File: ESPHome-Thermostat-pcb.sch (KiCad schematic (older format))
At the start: 97 parts, among them J1 Si7021, J2 MT3608, J3 Relay_Out, J4 SSD1306_Display, J5 Vin, Q1 NMOS_YJL03N06A, Q10 PMOS_AP40P05, Q11 NMOS_YJL03N06A, Q12 PMOS_AP40P05, Q13 PMOS_AP40P05, Q14 NMOS_YJL03N06A, Q15 NMOS_YJL03N06A, Q16 PMOS_AP40P05, Q17 NMOS_YJL03N06A, Q18 PMOS_AP40P05, Q19 PMOS_AP40P05, Q2 NMOS_YJL03N06A, Q20 PMOS_AP40P05, Q3 PMOS_AP40P05, Q4 PMOS_AP40P05, Q5 NMOS_YJL03N06A, Q6 NMOS_YJL03N06A, Q7 PMOS_AP40P05, Q8 PMOS_AP40P05, Q9 NMOS_YJL03N06A, SW1 EC11_Rotary_Encoder_Switch, U1 NodeMCU_1.0_(ESP-12E), U2 PCF8574, U3 AMS1117-3.3

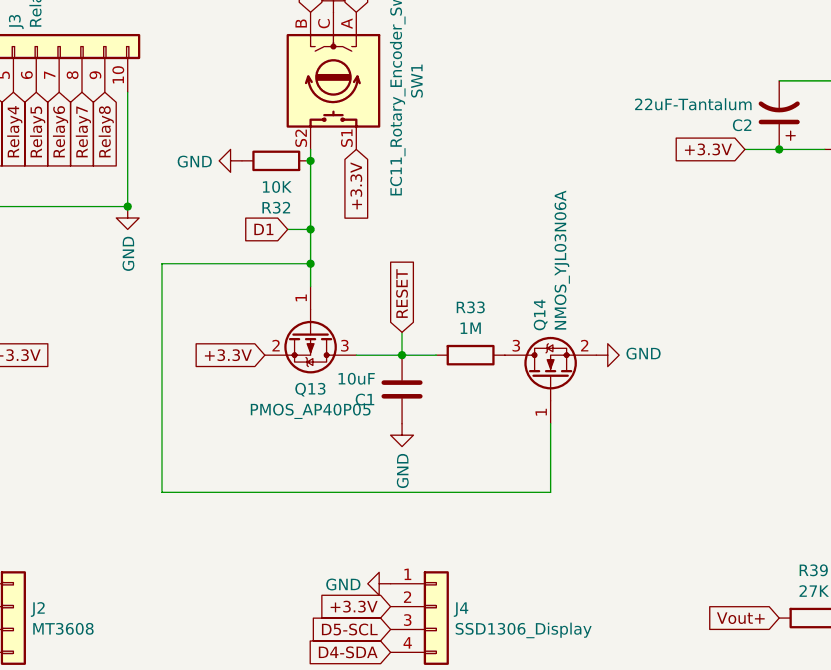
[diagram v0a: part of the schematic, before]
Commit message: development
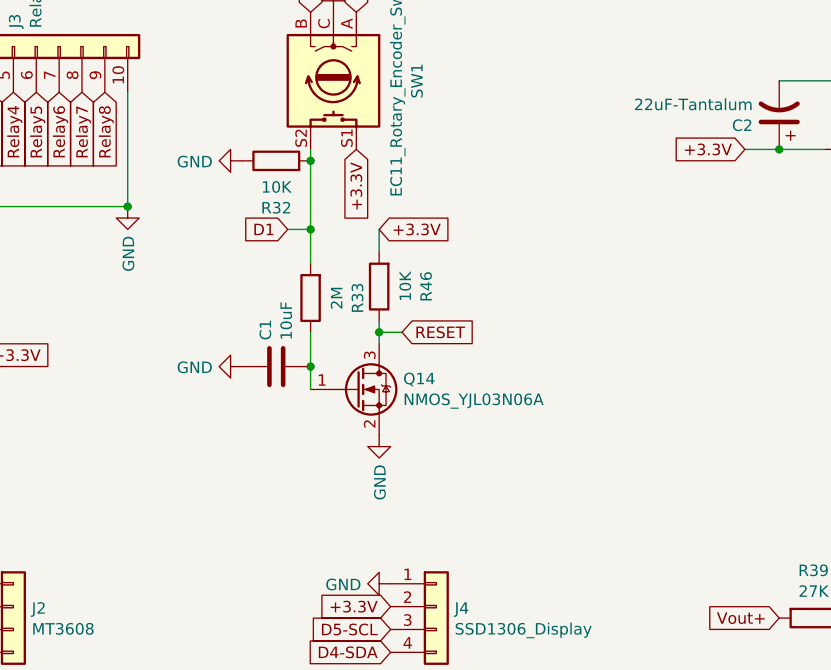
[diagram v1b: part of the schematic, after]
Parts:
- removed Q13: PMOS_AP40P05, Package_TO_SOT_SMD:SOT-23, symbol Device:Q_PMOS_GSD
- added R46: 10K, Resistor_SMD:R_0805_2012Metric, symbol Device:R
- R33: value 1M -> 2M
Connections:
- net +3.3V: now also R46.2
- net D1: now also R33.2; no longer Q14.1 (G)
- net RESET: now also Q14.3 (D), R46.1; no longer C1.2, R33.2
- net at R33.1: now also C1.2, Q14.1 (G); no longer Q14.3 (D)
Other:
- moved on the sheet: C1, Q14, R33
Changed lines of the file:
@@
 L Device:Q_NMOS_GSD Q14
 U 1 1 61CAFC02
-P 7750 2400
-F 0 "Q14" H 7955 2446 50  0000 L CNN
-F 1 "NMOS_YJL03N06A" H 7955 2355 50  0000 L CNN
-F 2 "Package_TO_SOT_SMD:SOT-23" H 7950 2500 50  0001 C CNN
-F 3 "~" H 7750 2400 50  0001 C CNN
-	1    7750 2400
-	0    -1   -1   0
+P 6900 2450
+F 0 "Q14" H 7105 2496 50  0000 L CNN
+F 1 "NMOS_YJL03N06A" H 7105 2405 50  0000 L CNN
+F 2 "Package_TO_SOT_SMD:SOT-23" H 7100 2550 50  0001 C CNN
+F 3 "~" H 6900 2450 50  0001 C CNN
+	1    6900 2450
+	1    0    0    -1
 $EndComp
 Wire Wire Line
@@
 Text GLabel 850  2250 0    50   Input ~ 0
 RESET
-$Comp
-L Device:Q_PMOS_GSD Q13
-U 1 1 61E18905
-P 6700 2200
-F 0 "Q13" V 6949 2200 50  0000 C CNN
-F 1 "PMOS_AP40P05" V 7040 2200 50  0000 C CNN
-F 2 "Package_TO_SOT_SMD:SOT-23" H 6900 2300 50  0001 C CNN
-F 3 "~" H 6700 2200 50  0001 C CNN
-	1    6700 2200
-	0    1    1    0
-$EndComp
-Text GLabel 6500 2300 0    50   Input ~ 0
-+3.3V
-Connection ~ 6700 1750
-Wire Wire Line
-	7100 2300 6900 2300
+Text GLabel 7000 1750 2    50   Input ~ 0
++3.3V
 $Comp
 L power:GND #PWR036
 U 1 1 61E9C208
-P 7100 2600
-F 0 "#PWR036" H 7100 2350 50  0001 C CNN
-F 1 "GND" V 7105 2472 50  0000 R CNN
-F 2 "" H 7100 2600 50  0001 C CNN
-F 3 "" H 7100 2600 50  0001 C CNN
-	1    7100 2600
-	1    0    0    -1
-$EndComp
-Text GLabel 7100 2200 1    50   Input ~ 0
+P 6400 2350
+F 0 "#PWR036" H 6400 2100 50  0001 C CNN
+F 1 "GND" V 6405 2222 50  0000 R CNN
+F 2 "" H 6400 2350 50  0001 C CNN
+F 3 "" H 6400 2350 50  0001 C CNN
+	1    6400 2350
+	0    1    1    0
+$EndComp
+Text GLabel 7100 2200 2    50   Input ~ 0
 RESET
-Wire Wire Line
-	7100 2200 7100 2300
-Connection ~ 7100 2300
 $Comp
 L Device:R R33
 U 1 1 61E9FC38
-P 7400 2300
-F 0 "R33" V 7193 2300 50  0000 C CNN
-F 1 "1M" V 7284 2300 50  0000 C CNN
-F 2 "Resistor_SMD:R_0805_2012Metric" V 7330 2300 50  0001 C CNN
-F 3 "~" H 7400 2300 50  0001 C CNN
-	1    7400 2300
-	0    1    1    0
-$EndComp
-Wire Wire Line
-	7250 2300 7100 2300
+P 6700 2050
+F 0 "R33" V 6493 2050 50  0000 C CNN
+F 1 "2M" V 6584 2050 50  0000 C CNN
+F 2 "Resistor_SMD:R_0805_2012Metric" V 6630 2050 50  0001 C CNN
+F 3 "~" H 6700 2050 50  0001 C CNN
+	1    6700 2050
+	-1   0    0    1
+$EndComp
 $Comp
 L power:GND #PWR038
 U 1 1 61EADD37
-P 7950 2300
-F 0 "#PWR038" H 7950 2050 50  0001 C CNN
-F 1 "GND" V 7955 2172 50  0000 R CNN
-F 2 "" H 7950 2300 50  0001 C CNN
-F 3 "" H 7950 2300 50  0001 C CNN
-	1    7950 2300
-	0    -1   -1   0
-$EndComp
-Wire Wire Line
-	6700 1750 6700 1900
-Wire Wire Line
-	7750 2600 7750 2900
-Wire Wire Line
-	7750 2900 6050 2900
-Wire Wire Line
-	6050 2900 6050 1900
-Wire Wire Line
-	6050 1900 6700 1900
-Connection ~ 6700 1900
-Wire Wire Line
-	6700 1900 6700 2000
+P 7000 2650
+F 0 "#PWR038" H 7000 2400 50  0001 C CNN
+F 1 "GND" V 7005 2522 50  0000 R CNN
+F 2 "" H 7000 2650 50  0001 C CNN
+F 3 "" H 7000 2650 50  0001 C CNN
+	1    7000 2650
+	1    0    0    -1
+$EndComp
 Wire Wire Line
 	2050 5200 2100 5200
@@
 L Device:C C1
 U 1 1 61D298D5
-P 7100 2450
-F 0 "C1" H 7215 2496 50  0000 L CNN
-F 1 "10uF" H 7215 2405 50  0000 L CNN
-F 2 "Capacitor_SMD:C_0805_2012Metric" H 7138 2300 50  0001 C CNN
-F 3 "~" H 7100 2450 50  0001 C CNN
-	1    7100 2450
-	-1   0    0    1
+P 6550 2350
+F 0 "C1" H 6665 2396 50  0000 L CNN
+F 1 "10uF" H 6665 2305 50  0000 L CNN
+F 2 "Capacitor_SMD:C_0805_2012Metric" H 6588 2200 50  0001 C CNN
+F 3 "~" H 6550 2350 50  0001 C CNN
+	1    6550 2350
+	0    -1   -1   0
 $EndComp
 Text GLabel 5000 1950 2    50   Input ~ 0
@@
 Wire Wire Line
 	5000 1850 5000 1950
+Wire Wire Line
+	6700 1900 6700 1750
+Connection ~ 6700 1750
+Wire Wire Line
+	6700 2200 6700 2350
+Connection ~ 6700 2350
+Wire Wire Line
+	6700 2350 6700 2450
+$Comp
+L Device:R R46
+U 1 1 61DFB003
+P 7000 2000
+F 0 "R46" V 6793 2000 50  0000 C CNN
+F 1 "10K" V 6884 2000 50  0000 C CNN
+F 2 "Resistor_SMD:R_0805_2012Metric" V 6930 2000 50  0001 C CNN
+F 3 "~" H 7000 2000 50  0001 C CNN
+	1    7000 2000
+	-1   0    0    1
+$EndComp
+Wire Wire Line
+	7000 1850 7000 1750
+Wire Wire Line
+	7000 2150 7000 2200
+Wire Wire Line
+	7100 2200 7000 2200
+Connection ~ 7000 2200
+Wire Wire Line
+	7000 2200 7000 2250
 $EndSCHEMATC
